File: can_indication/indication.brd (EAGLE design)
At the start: 69.9 x 63.5 mm, 31 parts, among them IC1 TPS92630QPWPRQ1, IC2 TPS92630QPWPRQ1

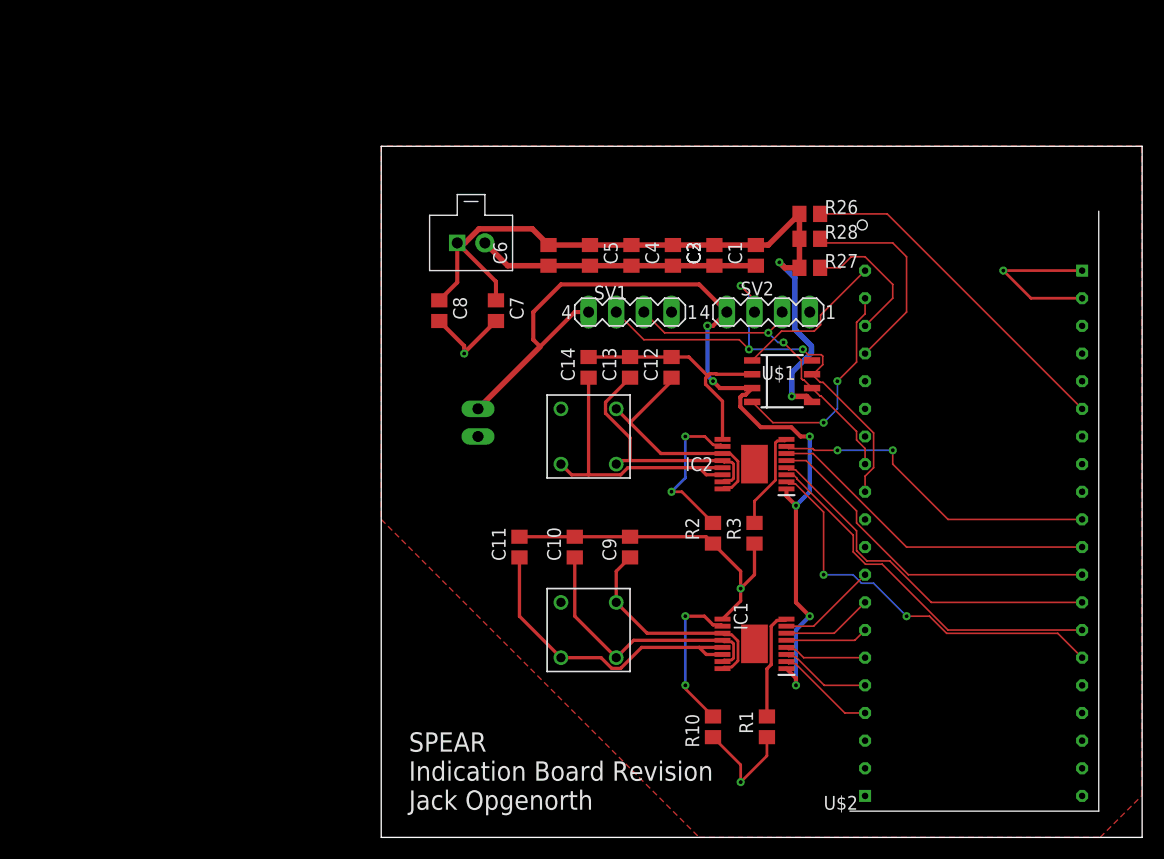
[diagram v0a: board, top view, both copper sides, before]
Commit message: new design to fix a bunch of problems
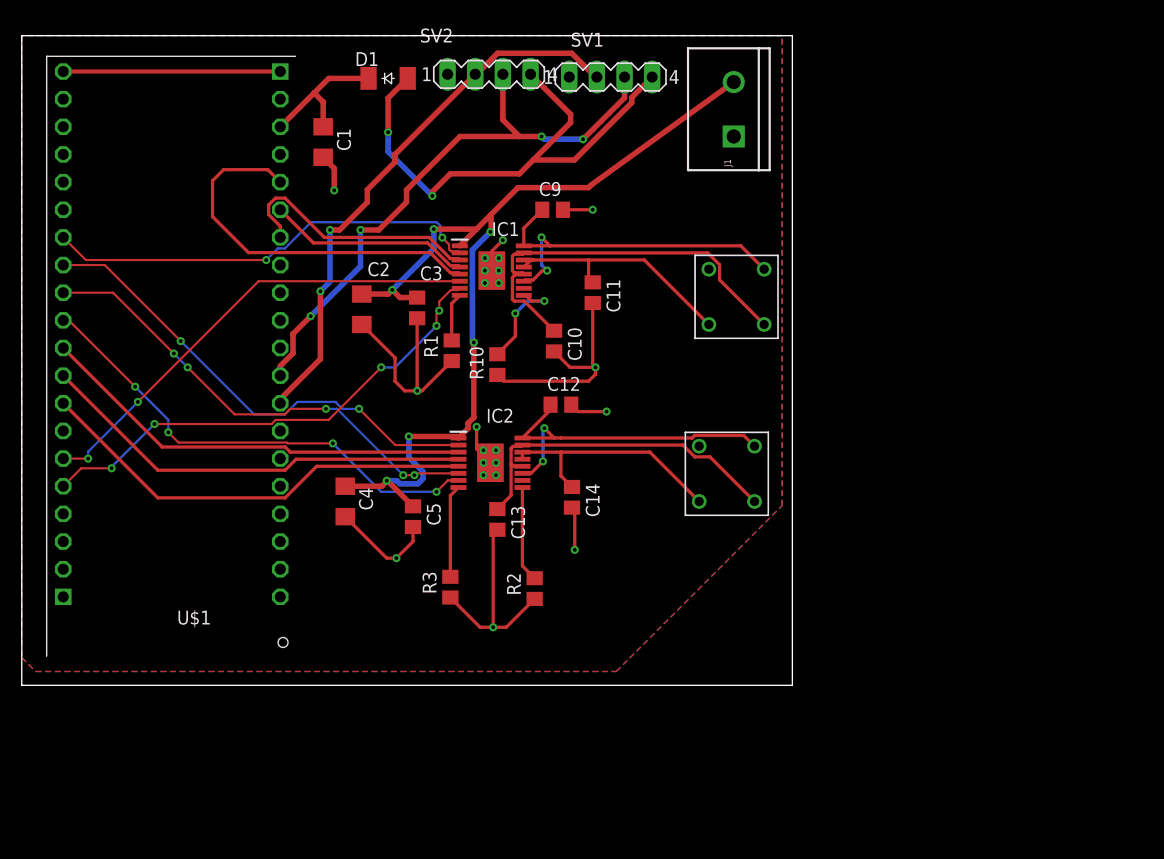
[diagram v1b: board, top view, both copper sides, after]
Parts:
- removed C6: 4u7, resistor:C0805
- removed C7: 10n, resistor:C0805
- removed C8: 1u, resistor:C0805
- removed JP1: (no value), pinhead:1X02
- removed R26, R27, R28: 10k, resistor:R0805
- removed U$2: STM-DEV-BOARD, SPEAR:STM-DEV-BOARD
- removed U$4: TE-CONN_5-103669-1, SPEAR:TE-CONN_5-103669-1
- added D1: CGRM4001-G, diode:SOD-123_MINI-SMA
- added J1: (no value), SparkFun-Connectors:SCREWTERMINAL-5MM-2
- C1: value 100n -> 100nf; device resistor:C0805 -> resistor:C1206
- C10, C11, C12, C13, C14, C9: value 100n -> 10n
- C2, C4: value 100n -> 10uF; device resistor:C0805 -> rcl:C1206
- C3, C5: value 100n -> 100nF; device resistor:C0805 -> rcl:C0805
- R1, R3: value 10K -> 100
- R10, R2: value 815 -> 2.5k
- U$1: value MCP2562-E/SN -> STM-DEV-BOARD; device SPEAR:SOIC8 -> SPEAR:STM-DEV-BOARD
- moved U$1 54.2 mm to (23.7, 78.0), turned to 180 degrees
- moved R1 45.1 mm to (39.5, 52.3)
- moved IC1 41.9 mm to (43.2, 59.7), turned to 0 degrees
- moved C1 41.1 mm to (27.7, 71.5)
- moved R10 38.7 mm to (43.7, 51.1)
- moved C4 34.7 mm to (29.7, 38.5)
- moved SV2 33.7 mm to (42.9, 77.7), turned to 0 degrees
- moved U$3 33.5 mm to (61.8, 53.5)
- moved C2 32.8 mm to (31.2, 56.1)
- moved C9 31.8 mm to (48.8, 65.3), turned to 0 degrees
- moved C5 29.0 mm to (35.9, 37.1)
- moved R3 28.4 mm to (39.4, 30.6)
- moved C11 24.3 mm to (52.5, 57.7), turned to 270 degrees
- moved IC2 24.3 mm to (43.1, 42.0), turned to 0 degrees
- moved C3 24.0 mm to (36.3, 56.3)
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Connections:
- removed net +5V: IC1.1, IC2.1, JP1.1, SV1.4, SV2.4, U$1.3
- removed net CAN_STBY: U$1.8
- removed net I2C_SCL: R27.1, U$2.PB14
- removed net I2C_SDA: R28.1, U$2.PB15
- removed net LED_!OE: R26.1, U$2.PB10
- removed net PA1: IC2.2, U$2.PA1
- removed net PA2: IC2.3, U$2.PA2
- removed net PA3: IC2.4, U$2.PA3
- removed net PA4: IC2.5, U$2.PA4
- removed net PA5: IC2.6, U$2.PA5
- removed net PA6: IC2.7, U$2.PA6
- removed net PB4: IC1.7, U$2.PB4
- removed net PB5: IC1.6, U$2.PB5
- removed net PB6: IC1.5, U$2.PB6
- removed net PB7: IC1.4, U$2.PB7
- removed net PB8: IC1.3, U$2.PB8
- removed net PB9: IC1.2, U$2.PB9
- removed net STM_CANRX: U$1.4, U$2.PB13
- removed net STM_CANTX: U$1.1, U$2.PB12
- new net 5V: C1.1, D1.C, U$1.5V
- new net EN1: IC1.2, U$1.PA2
- new net EN2: IC2.2, U$1.PA3
- new net FAULT1: IC1.6, U$1.PB10
- new net FAULT2: IC2.6, U$1.PA4
- new net FAULTS1: IC1.7, U$1.PB11
- new net FAULTS2: IC2.7, U$1.PA5
- new net N$4: D1.A, SV1.4, SV2.4
- new net TIM3_CH1: IC2.3, U$1.PA6
- new net TIM3_CH2: IC2.4, U$1.PA7
- new net TIM3_CH3: IC2.5, U$1.PB0
- new net TIM4_CH1: IC1.3, U$1.PB6
- new net TIM4_CH2: IC1.4, U$1.PB7
- new net TIM4_CH3: IC1.5, U$1.PB8
- new net VIN: C2.1, C3.1, C4.1, C5.1, IC1.1, IC2.1, J1.2
- net +3V3: now also U$1.3.3V, U$1.VBAT; no longer C1.1, C2.1, C3.1, C4.1, C5.1, C6.1, C7.1, C8.1, R26.2, R27.2, R28.2, U$1.5, U$4.P$1
- net CANH: now also U$1.CANH; no longer U$1.7, U$2.CANH
- net CANL: now also U$1.CANL; no longer U$1.6, U$2.CANL
- net GND: now also IC1.10, IC1.17, IC2.10, IC2.17, J1.1, U$1.GND, U$1.GND@2, U$1.GND@3; no longer C6.2, C7.2, C8.2, IC1.9, IC2.9, JP1.2, U$1.2, U$2.GND@2, U$2.GND@3, U$4.P$2
- net N$1: now also IC1.9; no longer IC1.10
- net N$3: now also IC2.9; no longer IC2.10
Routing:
- net VIN: track 0.00 -> 89.2 mm, vias 0 -> 6
- net +5V: track 86.7 -> 0.00 mm, vias 6 -> 0
- net +3V3: track 69.8 -> 19.9 mm, vias 2 -> 0
- net N$4: track 0.00 -> 49.7 mm, vias 0 -> 2
- net FAULTS1: track 0.00 -> 45.2 mm, vias 0 -> 5
- net EN2: track 0.00 -> 44.1 mm, vias 0 -> 2
- net FAULTS2: track 0.00 -> 43.9 mm, vias 0 -> 4
- net FAULT2: track 0.00 -> 43.7 mm, vias 0 -> 5
- net FAULT1: track 0.00 -> 43.6 mm, vias 0 -> 2
- net TIM3_CH3: track 0.00 -> 41.1 mm
- net EN1: track 0.00 -> 40.7 mm, vias 0 -> 2
- net TIM3_CH2: track 0.00 -> 40.3 mm
- net TIM3_CH1: track 0.00 -> 40.3 mm
- net PA1: track 37.2 -> 0.00 mm, vias 2 -> 0
- net TIM4_CH3: track 0.00 -> 35.3 mm
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- added copper zone on layer 16, net GND
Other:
- board size 69.9 x 63.5 mm -> 70.8 x 59.7 mm
- board text removed: "SPEAR Indication Board Revision Jack Opgenorth"
